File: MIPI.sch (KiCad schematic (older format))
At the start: 40 parts, among them J8 49F-1201GYD2NL, U1 AllWinner-S3(FBGA-234), Y2 32.768kHz, Y3 24MHz

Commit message: OtterCastAmp inital commit
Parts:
- J8: symbol otter:49F-1201GYD2NL -> OtterCastAmp-rescue:49F-1201GYD2NL-otter
- U1: symbol otter:AllWinner-S3(FBGA-234) -> OtterCastAmp-rescue:AllWinner-S3(FBGA-234)-otter
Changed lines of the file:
@@
 	2700 1900 2300 1900
 $Comp
-L S3-OLinuXino_Rev_A:GND #PWR?
+L OtterCastAmp-rescue:GND-S3-OLinuXino_Rev_A #PWR?
 U 1 1 621FAA13
 P 2000 1900
@@
 $EndComp
 $Comp
-L S3-OLinuXino_Rev_A:GND #PWR?
+L OtterCastAmp-rescue:GND-S3-OLinuXino_Rev_A #PWR?
 U 1 1 621FAA25
 P 2350 3900
@@
 $EndComp
 $Comp
-L S3-OLinuXino_Rev_A:+3.0VA #PWR?
+L OtterCastAmp-rescue:+3.0VA-S3-OLinuXino_Rev_A #PWR?
 U 1 1 621FAA2B
 P 2350 3700
@@
 $EndComp
 $Comp
-L S3-OLinuXino_Rev_A:+3.3V #PWR?
+L OtterCastAmp-rescue:+3.3V-S3-OLinuXino_Rev_A #PWR?
 U 1 1 621FAA43
 P 1900 2300
@@
 $EndComp
 $Comp
-L S3-OLinuXino_Rev_A:GND #PWR?
+L OtterCastAmp-rescue:GND-S3-OLinuXino_Rev_A #PWR?
 U 1 1 621FAA8A
 P 1200 4350
@@
 $EndComp
 $Comp
-L S3-OLinuXino_Rev_A:GND #PWR?
+L OtterCastAmp-rescue:GND-S3-OLinuXino_Rev_A #PWR?
 U 1 1 621FAA9B
 P 1550 4500
@@
 $EndComp
 $Comp
-L S3-OLinuXino_Rev_A:+3.3V #PWR?
+L OtterCastAmp-rescue:+3.3V-S3-OLinuXino_Rev_A #PWR?
 U 1 1 621FAAB0
 P 1200 4100
@@
 $EndComp
 $Comp
-L S3-OLinuXino_Rev_A:GND #PWR?
+L OtterCastAmp-rescue:GND-S3-OLinuXino_Rev_A #PWR?
 U 1 1 621FAAC7
 P 2550 5650
@@
 $EndComp
 $Comp
-L S3-OLinuXino_Rev_A:VCC-DDR #PWR?
+L OtterCastAmp-rescue:VCC-DDR-S3-OLinuXino_Rev_A #PWR?
 U 1 1 621FAAD2
 P 1550 4750
@@
 	2500 5200 2700 5200
 $Comp
-L S3-OLinuXino_Rev_A:GND #PWR?
+L OtterCastAmp-rescue:GND-S3-OLinuXino_Rev_A #PWR?
 U 1 1 621FAAF3
 P 2150 5400
@@
 $EndComp
 $Comp
-L S3-OLinuXino_Rev_A:+3.0VA #PWR?
+L OtterCastAmp-rescue:+3.0VA-S3-OLinuXino_Rev_A #PWR?
 U 1 1 621FAB39
 P 5950 5000
@@
 	4100 4400 4550 4400
 $Comp
-L S3-OLinuXino_Rev_A:GND #PWR?
+L OtterCastAmp-rescue:GND-S3-OLinuXino_Rev_A #PWR?
 U 1 1 621FAB92
 P 4800 3800
@@
 $EndComp
 $Comp
-L S3-OLinuXino_Rev_A:GND #PWR?
+L OtterCastAmp-rescue:GND-S3-OLinuXino_Rev_A #PWR?
 U 1 1 621FAB9A
 P 5350 3700
@@
 $EndComp
 $Comp
-L S3-OLinuXino_Rev_A:+3.3V #PWR?
+L OtterCastAmp-rescue:+3.3V-S3-OLinuXino_Rev_A #PWR?
 U 1 1 621FABA1
 P 5350 3400
@@
 $EndComp
 $Comp
-L S3-OLinuXino_Rev_A:+1.1V #PWRV?
+L OtterCastAmp-rescue:+1.1V-S3-OLinuXino_Rev_A #PWRV?
 U 1 1 621FABBF
 P 4800 3500
@@
 $EndComp
 $Comp
-L S3-OLinuXino_Rev_A:+3.3V_RTC #PWR?
+L OtterCastAmp-rescue:+3.3V_RTC-S3-OLinuXino_Rev_A #PWR?
 U 1 1 621FAC6A
 P 5950 4350
@@
 $EndComp
 $Comp
-L S3-OLinuXino_Rev_A:+3.3V #PWR?
+L OtterCastAmp-rescue:+3.3V-S3-OLinuXino_Rev_A #PWR?
 U 1 1 621FACF7
 P 4100 2200
@@
 $EndComp
 $Comp
-L otter:AllWinner-S3(FBGA-234) U?
+L OtterCastAmp-rescue:AllWinner-S3(FBGA-234)-otter U?
 U 5 1 67B22B9C
 P 3400 3600
@@
 	1150 3800 1150 3750
 $Comp
-L S3-OLinuXino_Rev_A:GND #PWR?
+L OtterCastAmp-rescue:GND-S3-OLinuXino_Rev_A #PWR?
 U 1 1 682228FC
 P 1100 3800
@@
 	4400 5200 4100 5200
 $Comp
-L S3-OLinuXino_Rev_A:GND #PWR?
+L OtterCastAmp-rescue:GND-S3-OLinuXino_Rev_A #PWR?
 U 1 1 68801614
 P 4600 5250
@@
 Connection ~ 4700 5150
 $Comp
-L S3-OLinuXino_Rev_A:GND #PWR?
+L OtterCastAmp-rescue:GND-S3-OLinuXino_Rev_A #PWR?
 U 1 1 6887244B
 P 4800 5250
@@
 	4700 5150 5050 5150
 $Comp
-L S3-OLinuXino_Rev_A:GND #PWR?
+L OtterCastAmp-rescue:GND-S3-OLinuXino_Rev_A #PWR?
 U 1 1 688B7D1F
 P 5350 5350
@@
 	5350 5350 5250 5350
 $Comp
-L S3-OLinuXino_Rev_A:GND #PWR?
+L OtterCastAmp-rescue:GND-S3-OLinuXino_Rev_A #PWR?
 U 1 1 688D2E39
 P 5350 5150
@@
 	5350 5150 5250 5150
 $Comp
-L S3-OLinuXino_Rev_A:GND #PWR?
+L OtterCastAmp-rescue:GND-S3-OLinuXino_Rev_A #PWR?
 U 1 1 688E06D9
 P 5950 5300
@@
 $EndComp
 $Comp
-L S3-OLinuXino_Rev_A:GND #PWR?
+L OtterCastAmp-rescue:GND-S3-OLinuXino_Rev_A #PWR?
 U 1 1 68934D4E
 P 4700 4900
@@
 $EndComp
 $Comp
-L S3-OLinuXino_Rev_A:GND #PWR?
+L OtterCastAmp-rescue:GND-S3-OLinuXino_Rev_A #PWR?
 U 1 1 6898A97A
 P 5550 4800
@@
 	5550 4800 5450 4800
 $Comp
-L S3-OLinuXino_Rev_A:GND #PWR?
+L OtterCastAmp-rescue:GND-S3-OLinuXino_Rev_A #PWR?
 U 1 1 6898A981
 P 5550 4600
@@
 	5950 4450 5950 4400
 $Comp
-L S3-OLinuXino_Rev_A:GND #PWR?
+L OtterCastAmp-rescue:GND-S3-OLinuXino_Rev_A #PWR?
 U 1 1 68A05AC3
 P 5950 4650
@@
 EPHY_SPD_LED
 $Comp
-L S3-OLinuXino_Rev_A:+3.3V #PWR?
+L OtterCastAmp-rescue:+3.3V-S3-OLinuXino_Rev_A #PWR?
 U 1 1 68ABBB53
 P 7750 1650
@@
 $EndComp
 $Comp
-L S3-OLinuXino_Rev_A:+3.3V #PWR?
+L OtterCastAmp-rescue:+3.3V-S3-OLinuXino_Rev_A #PWR?
 U 1 1 68AC8602
 P 7450 1650
@@
 $EndComp
 $Comp
-L S3-OLinuXino_Rev_A:GND #PWR?
+L OtterCastAmp-rescue:GND-S3-OLinuXino_Rev_A #PWR?
 U 1 1 68B013CC
 P 8450 2500
@@
 $EndComp
 $Comp
-L S3-OLinuXino_Rev_A:GND #PWR?
+L OtterCastAmp-rescue:GND-S3-OLinuXino_Rev_A #PWR?
 U 1 1 68B0DC25
 P 8450 2100
@@
 	8950 2250 9000 2250
 $Comp
-L S3-OLinuXino_Rev_A:GND #PWR?
+L OtterCastAmp-rescue:GND-S3-OLinuXino_Rev_A #PWR?
 U 1 1 68C73D5E
 P 9700 2100
@@
 $EndComp
 $Comp
-L S3-OLinuXino_Rev_A:GND #PWR?
+L OtterCastAmp-rescue:GND-S3-OLinuXino_Rev_A #PWR?
 U 1 1 68C80600
 P 9700 2500
@@
 $EndComp
 $Comp
-L S3-OLinuXino_Rev_A:GND #PWR?
+L OtterCastAmp-rescue:GND-S3-OLinuXino_Rev_A #PWR?
 U 1 1 68C8FA66
 P 7550 3150
@@
 Connection ~ 1600 4750
 $Comp
-L S3-OLinuXino_Rev_A:GND #PWR?
+L OtterCastAmp-rescue:GND-S3-OLinuXino_Rev_A #PWR?
 U 1 1 68D50852
 P 1550 5100
@@
 	9350 2500 9350 2550
 $Comp
-L otter:49F-1201GYD2NL J8
+L OtterCastAmp-rescue:49F-1201GYD2NL-otter J8
 U 1 1 60475CA8
 P 7550 2300
@@
 	7350 1350 7350 1200
 $Comp
-L S3-OLinuXino_Rev_A:GND #PWR?
+L OtterCastAmp-rescue:GND-S3-OLinuXino_Rev_A #PWR?
 U 1 1 60388407
 P 5100 4200

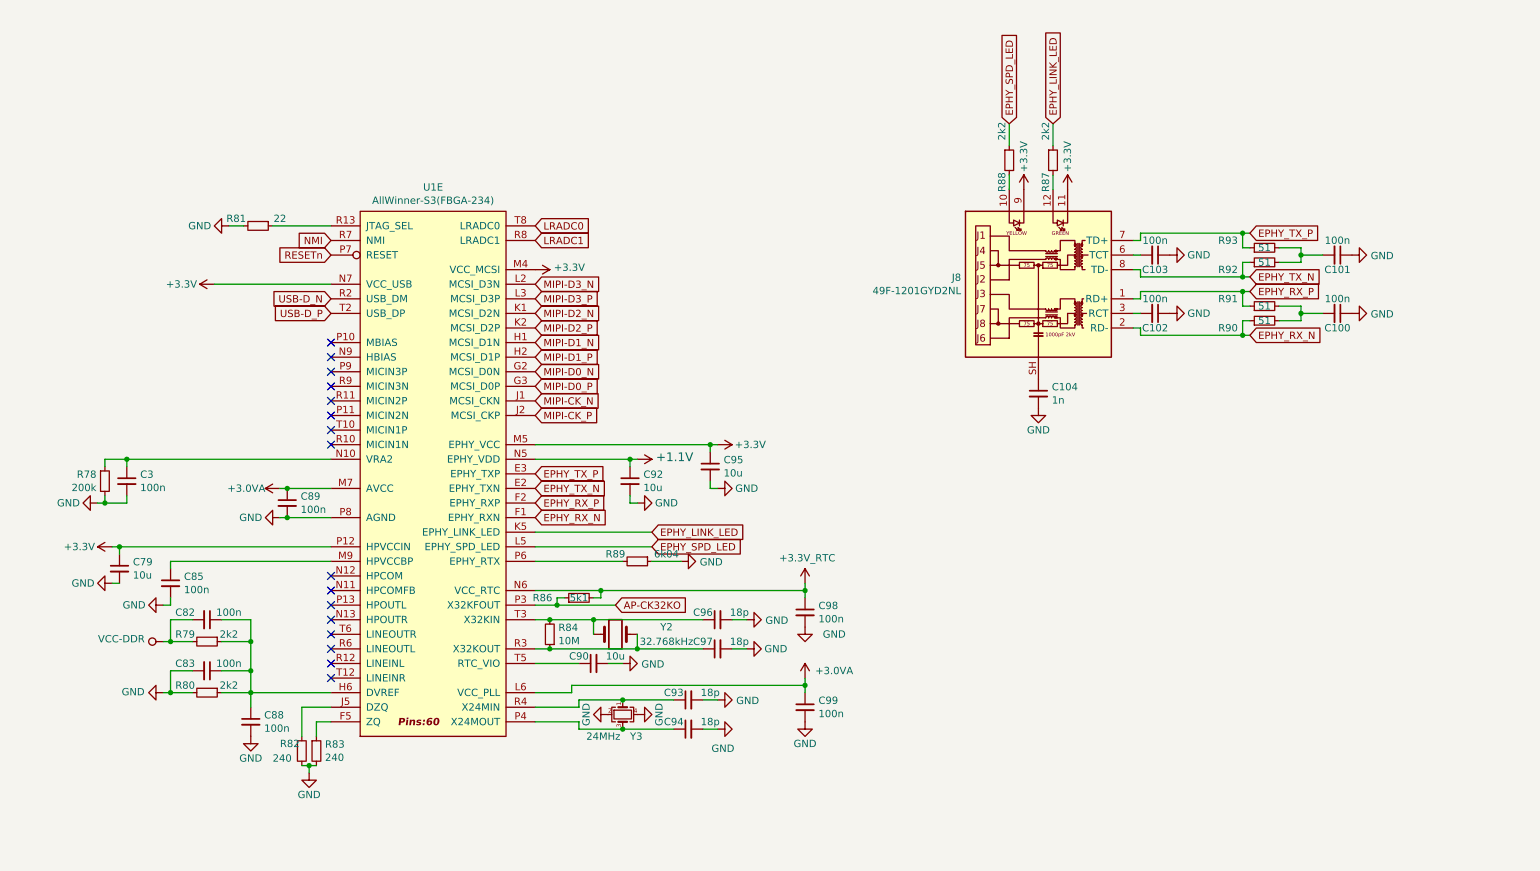
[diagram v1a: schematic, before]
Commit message: started layout
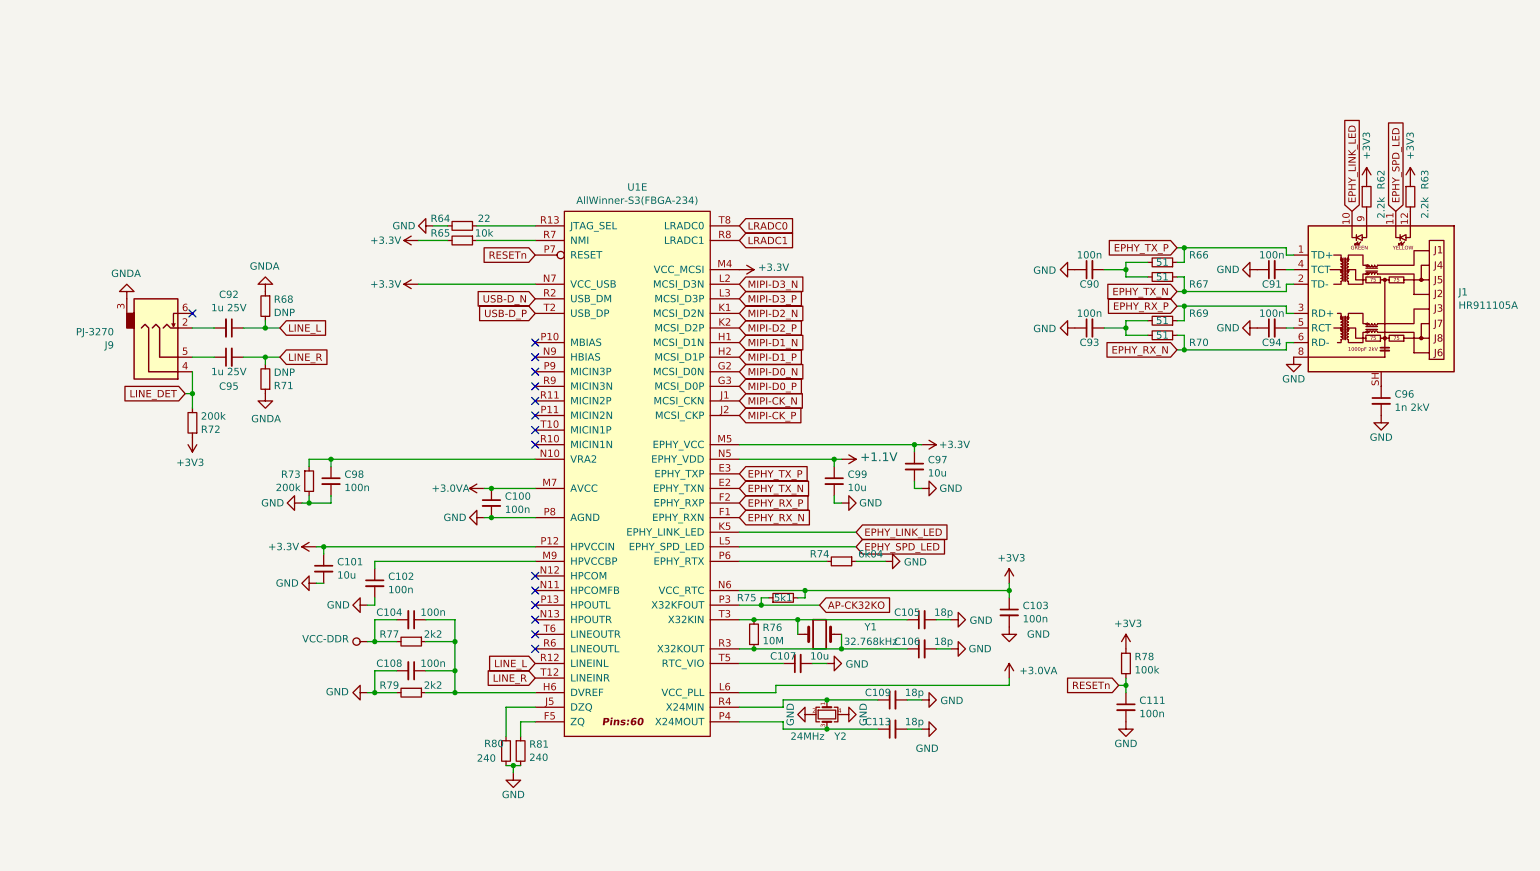
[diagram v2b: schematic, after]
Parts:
- removed C104: 1n, otter:C_0805, symbol Device:C_Small
- removed C88, C99: 100n, otter:C_0402, symbol Device:C_Small
- removed J8: 49F-1201GYD2NL, otter:49F-1201GYDXNL, symbol OtterCastAmp-rescue:49F-1201GYD2NL-otter
- removed R87, R88: 2k2, otter:R_0402, symbol Device:R_Small
- added C111: 100n, otter:C_0402, symbol Device:C_Small
- added C92, C95: 1u 25V, otter:C_0603, symbol Device:C_Small
- added C96: 1n 2kV, Capacitor_SMD:C_1206_3216Metric, symbol Device:C_Small
- added J1: HR911105A, Connector_RJ:RJ45_Hanrun_HR911105A, symbol otter:HR911105A
- added J9: PJ-3270, otter:PJ-3270, symbol OtterCastAmp-rescue:PJ-3270-otter
- added R62, R63: 2.2k, otter:R_0402, symbol Device:R_Small
- added R65: 10k, otter:R_0402, symbol Device:R_Small
- added R68, R71: DNP, otter:R_0402, symbol Device:R_Small
- added R72: 200k, otter:R_0402, symbol Device:R_Small
- added R78: 100k, otter:R_0402, symbol Device:R_Small
- renumbered C89 to C100, C79 to C101, C85 to C102, C98 to C103, C82 to C104, C96 to C105, C97 to C106, C90 to C107, C83 to C108, C93 to C109, C94 to C113, C101 to C90, C103 to C91, C100 to C93, C102 to C94, C95 to C97, C3 to C98, C92 to C99, R81 to R64, R93 to R66, R92 to R67, R91 to R69, R90 to R70, R78 to R73, R89 to R74, R86 to R75, R84 to R76, R79 to R77, R80 to R79, R82 to R80, R83 to R81, Y2 to Y1, Y3 to Y2
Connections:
- net +3.3V_RTC is gone; now on net +3V3: C103.1, R75.2, U1.N6 (VCC_RTC)
- net +3V3: now also R62.1, R63.1, R65.2, R72.1, R78.1
- net EPHY_LINK_LED: now also J1.10
- net EPHY_RX_N: now also J1.6 (RD-)
- net EPHY_RX_P: now also J1.3 (RD+)
- net EPHY_SPD_LED: now also J1.11
- net EPHY_TX_N: now also J1.2 (TD-)
- net EPHY_TX_P: now also J1.1 (TD+)
- net GND: now also C111.2, C96.2, J1.8
- net RESETn: now also C111.1, R78.2
- net at C94.2: now also J1.5 (RCT)
- net at C91.2: now also J1.4 (TCT)
- net LINE_L: now reaches U1.R12 (LINEINL)
- net LINE_L: now also C92.1, R68.2
- net LINE_R: now reaches U1.T12 (LINEINR)
- net LINE_R: now also C95.2, R71.2
- net NMI: no longer names the net of U1.R7 (NMI)
- net NMI: now also R65.1
- new net: J1.12, R63.2
- new net: J1.9, R62.2
- new net: C96.1, J1.SH
- new net: C92.2, J9.2
- new net: C95.1, J9.5
- new net GNDA: J9.3, R68.1, R71.1
- new net LINE_DET: J9.4, R72.2
- no-connect marks 16 -> 15
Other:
- moved on the sheet: C100, C101, C102, C103, C104, C105, C106, C107, C108, C109, C113, C90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

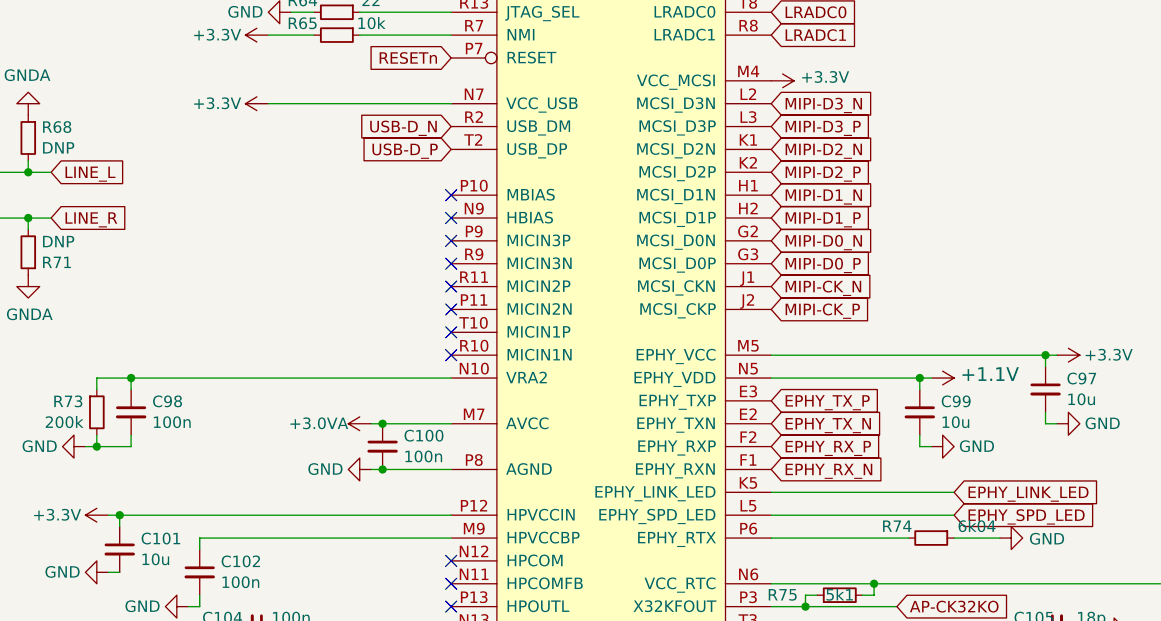
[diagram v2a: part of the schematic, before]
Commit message: layout final?
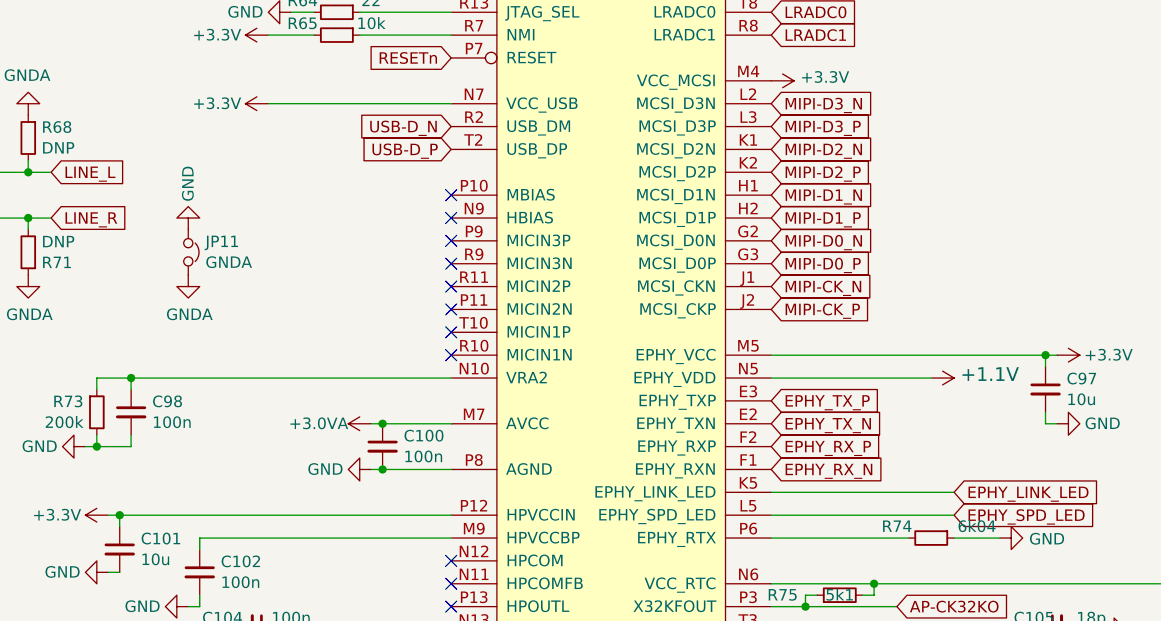
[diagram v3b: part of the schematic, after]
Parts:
- removed C99: 10u, otter:C_0603, symbol Device:C_Small
- added JP11: GNDA, Jumper:SolderJumper-2_P1.3mm_Bridged_Pad1.0x1.5mm, symbol Device:Jumper_NC_Small
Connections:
- net GND: now also JP11.1
- net GNDA: now also JP11.2
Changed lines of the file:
@@
-$Comp
-L OtterCastAmp-rescue:GND-S3-OLinuXino_Rev_A #PWR?
-U 1 1 621FAB92
-P 6200 3800
-AR Path="/5D8A1FAC/621FAB92" Ref="#PWR?"  Part="1"
-AR Path="/621FAB92" Ref="#PWR?"  Part="1"
-AR Path="/620E795B/621FAB92" Ref="#PWR0178"  Part="1"
-F 0 "#PWR0178" H 6200 3550 50  0001 C CNN
-F 1 "GND" V 6200 3600 50  0000 C CNN
-F 2 "" H 6200 3800 60  0000 C CNN
-F 3 "" H 6200 3800 60  0000 C CNN
-	1    6200 3800
-	0    -1   1    0
-$EndComp
 $Comp
 L OtterCastAmp-rescue:GND-S3-OLinuXino_Rev_A #PWR?
@@
 $Comp
 L Device:C_Small C?
-U 1 1 6843A0ED
-P 6150 3650
-AR Path="/6843A0ED" Ref="C?"  Part="1"
-AR Path="/602ACDF9/6843A0ED" Ref="C?"  Part="1"
-AR Path="/620E795B/6843A0ED" Ref="C99"  Part="1"
-F 0 "C99" H 6242 3696 50  0000 L CNN
-F 1 "10u" H 6242 3605 50  0000 L CNN
-F 2 "otter:C_0603" H 6150 3650 50  0001 C CNN
-F 3 "~" H 6150 3650 50  0001 C CNN
-	1    6150 3650
-	1    0    0    -1
-$EndComp
-$Comp
-L Device:C_Small C?
 U 1 1 684474E1
 P 6700 3550
@@
 $EndComp
 Wire Wire Line
-	6150 3500 6150 3550
-Wire Wire Line
 	6700 3400 6700 3450
-Wire Wire Line
-	5500 3500 6150 3500
 Wire Wire Line
 	6750 3400 6700 3400
 Connection ~ 6700 3400
-Wire Wire Line
-	6200 3500 6150 3500
-Connection ~ 6150 3500
-Wire Wire Line
-	6200 3800 6150 3800
-Wire Wire Line
-	6150 3800 6150 3750
 Wire Wire Line
 	6750 3700 6700 3700
@@
 $EndComp
 $Comp
-L power:+3V3 #PWR?
+L power:+3V3 #PWR0157
 U 1 1 60B95A7B
 P 7350 4350
-F 0 "#PWR?" H 7350 4200 50  0001 C CNN
+F 0 "#PWR0157" H 7350 4200 50  0001 C CNN
 F 1 "+3V3" H 7365 4523 50  0000 C CNN
 F 2 "" H 7350 4350 50  0001 C CNN
@@
 	1    0    0    -1
 $EndComp
+$Comp
+L power:GNDA #PWR?
+U 1 1 60D57C63
+P 2950 3050
+AR Path="/604A1CEE/60D57C63" Ref="#PWR?"  Part="1"
+AR Path="/620E795B/60D57C63" Ref="#PWR0251"  Part="1"
+F 0 "#PWR0251" H 2950 2800 50  0001 C CNN
+F 1 "GNDA" H 2955 2877 50  0000 C CNN
+F 2 "" H 2950 3050 50  0001 C CNN
+F 3 "" H 2950 3050 50  0001 C CNN
+	1    2950 3050
+	1    0    0    -1
+$EndComp
+$Comp
+L Device:Jumper_NC_Small JP11
+U 1 1 60D59415
+P 2950 2950
+F 0 "JP11" V 2904 3025 50  0000 L CNN
+F 1 "GNDA" V 2995 3025 50  0000 L CNN
+F 2 "Jumper:SolderJumper-2_P1.3mm_Bridged_Pad1.0x1.5mm" H 2950 2950 50  0001 C CNN
+F 3 "~" H 2950 2950 50  0001 C CNN
+	1    2950 2950
+	0    1    1    0
+$EndComp
+$Comp
+L OtterCastAmp-rescue:GND-S3-OLinuXino_Rev_A #PWR?
+U 1 1 60D59D85
+P 2950 2850
+AR Path="/5D8A1FAC/60D59D85" Ref="#PWR?"  Part="1"
+AR Path="/60D59D85" Ref="#PWR?"  Part="1"
+AR Path="/620E795B/60D59D85" Ref="#PWR0252"  Part="1"
+F 0 "#PWR0252" H 2950 2600 50  0001 C CNN
+F 1 "GND" V 2950 2650 50  0000 C CNN
+F 2 "" H 2950 2850 60  0000 C CNN
+F 3 "" H 2950 2850 60  0000 C CNN
+	1    2950 2850
+	1    0    0    1
+$EndComp
+Wire Wire Line
+	5500 3500 6200 3500
 $EndSCHEMATC
